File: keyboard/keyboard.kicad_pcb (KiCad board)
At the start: 2 copper layers, 210 parts, among them J1 Pico-EZmate, J3 Debug, K1 Esc, K10 F9, K11 F10, K12 F11, K13 F12, K15 ~~,`, K16 !,1, K17 @,2, K18 #,3, K19 $,4, K2 F1, K20 %,5, K21 ^,6, K22 &,7, K23 *,8, K24 (,9, K25 ),0, K26 _,-, K27 +,=, K28 Backspace, K29 Tab, K3 F2, K30 Q, K31 W, K32 E, K33 R, K34 T, K35 Y, K36 U, K37 I, K38 O, K39 P, K4 F3, K40 {,[, K41 },], K42 |,\, K43 Caps Lock, K44 A, K45 S, K46 D, K47 F, K48 G, K49 H, K5 F4, K50 J, K51 K, K52 L, K53 :,;, K54 ",', K55 Enter, K56 Shift, K57 Z, K58 X, K59 C, K6 F5, K60 V, K61 B, K62 N, K63 M, K64 <,,, K65 >,., K66 ?,/, K67 ↑, K68 Shift, K69 Fn, K7 F6, K70 Ctrl, K71 Alt, K72 Meta, K73 Space, K74 Space, K75 Meta, K76 Alt, K77 ←, K78 ↓, K79 →, K8 F7, K9 F8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

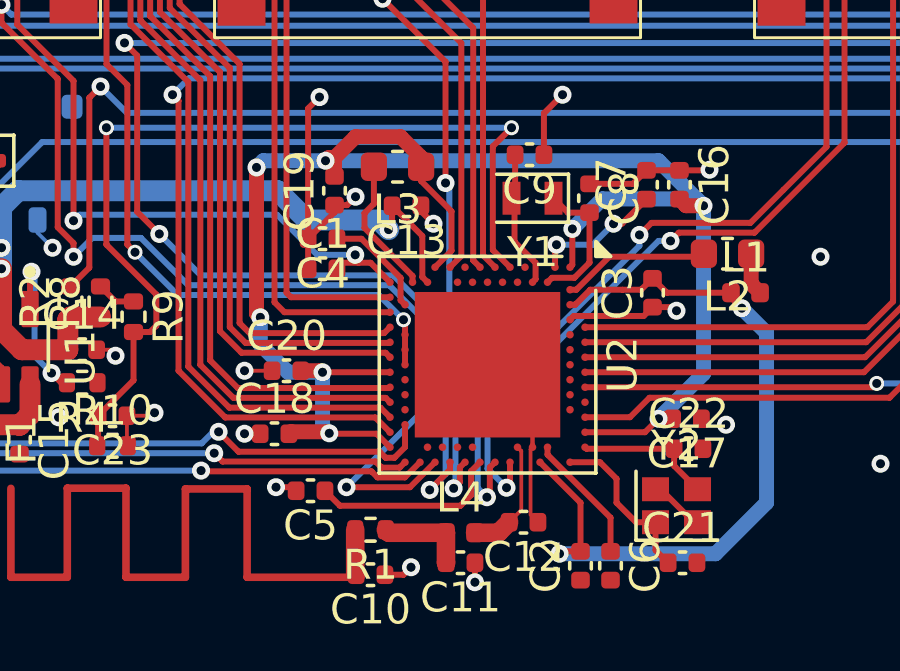
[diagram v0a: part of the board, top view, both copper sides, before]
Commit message: implemented most features
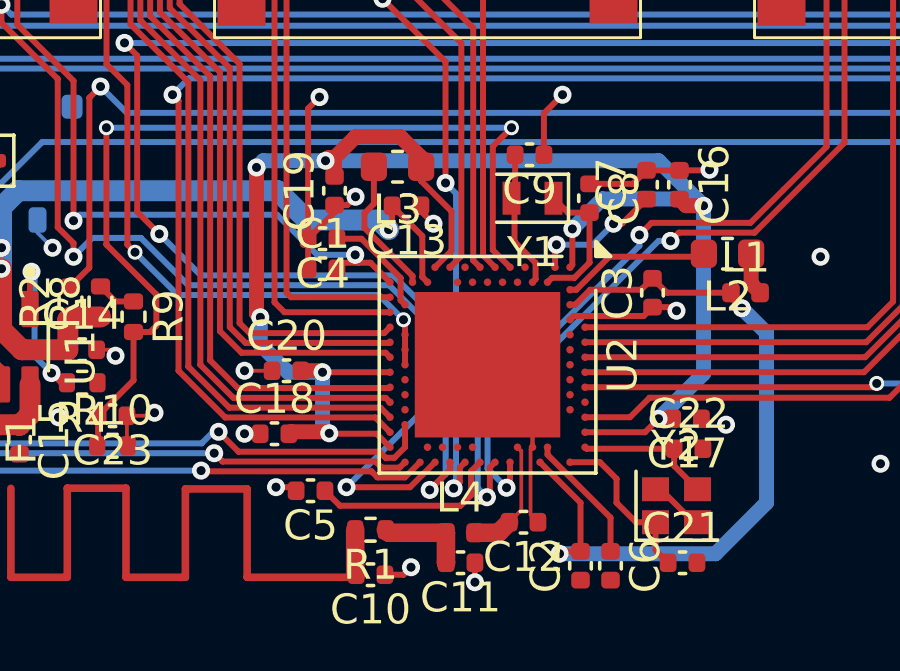
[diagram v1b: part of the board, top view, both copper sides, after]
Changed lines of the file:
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@@
+	)
+	(segment
+		(start 140.25 143.540581)
+		(end 140.25 133.792209)
+		(width 0.2)
+		(layer "B.Cu")
+		(net 44)
 	)
 	(segment
@@
 	)
 	(segment
-		(start 139.848737 137.751263)
-		(end 140.027 137.573)
-		(width 0.2)
-		(layer "B.Cu")
-		(net 44)
-	)
-	(segment
-		(start 140.027 133.569209)
-		(end 139.9 133.442209)
-		(width 0.2)
-		(layer "B.Cu")
-		(net 44)
-	)
-	(segment
 		(start 172.2 116.3)
 		(end 209.8 116.3)
@@
 	)
 	(segment
-		(start 140.232182 143.558399)
-		(end 140.232182 138.134708)
+		(start 140.17154 143.619041)
+		(end 140.25 143.540581)
 		(width 0.2)
 		(layer "B.Cu")
@@
 	)
 	(segment
-		(start 140.027 137.573)
-		(end 140.027 133.569209)
+		(start 140.25 133.792209)
+		(end 139.9 133.442209)
 		(width 0.2)
 		(layer "B.Cu")
@@
 		(width 0.2)
 		(layer "B.Cu")
-		(net 44)
-	)
-	(segment
-		(start 140.17154 143.619041)
-		(end 140.232182 143.558399)
-		(width 0.2)
-		(layer "B.Cu")
-		(net 44)
-	)
-	(segment
-		(start 140.232182 138.134708)
-		(end 139.848737 137.751263)
-		(width 0.2)
-		(layer "B.Cu")

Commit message: CAD work + documentation
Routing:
- net GND: track 30.3 -> 30.9 mm, vias 99 -> 104
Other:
- board outline added: 258.4 x 104.6 mm
